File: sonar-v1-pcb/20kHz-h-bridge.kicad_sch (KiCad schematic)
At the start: 1 part, among them U34 DRV8876PWPR

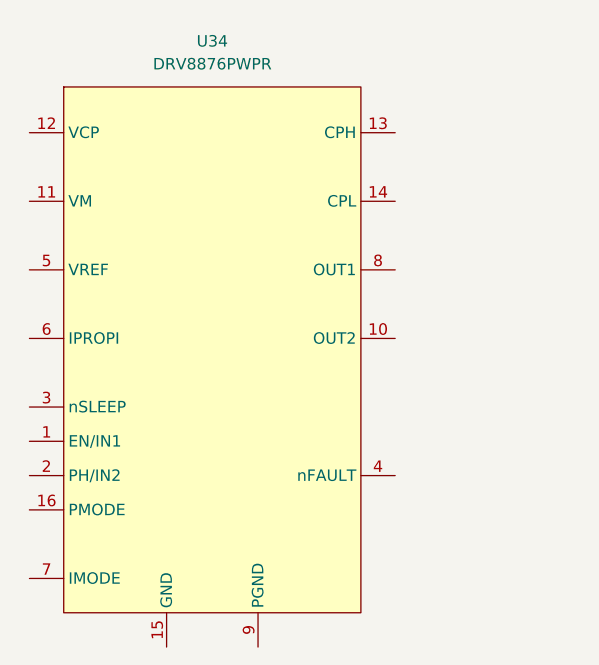
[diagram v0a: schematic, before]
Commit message: Do some power work
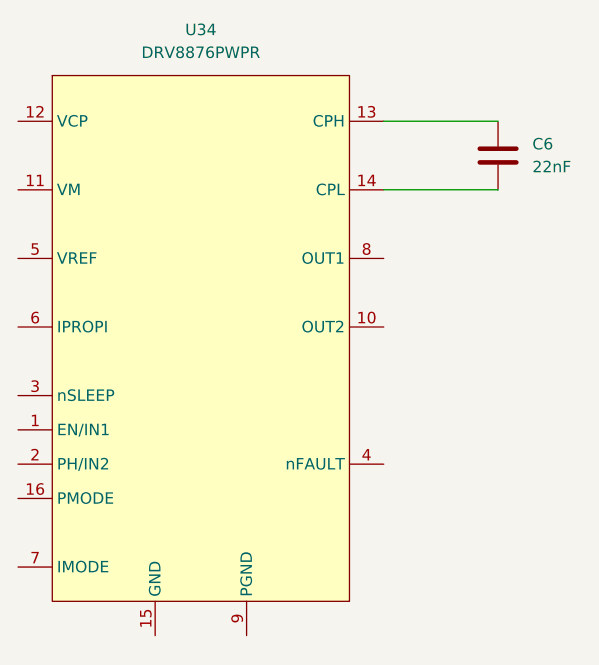
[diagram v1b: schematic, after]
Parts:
- added C6: 22nF, GS_Capacitors:C_0603_1608Metric, symbol GS_Capacitor_0603:C_0603_22nF
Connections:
- net at U34.13 (CPH): now also C6.1
- net at U34.14 (CPL): now also C6.2
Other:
- moved on the sheet: U34
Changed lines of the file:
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@@
 		(comment 1 "George Sleen")
+	)
+	(wire
+		(pts
+			(xy 180.34 86.36) (xy 167.64 86.36)
+		)
+		(stroke
+			(width 0)
+			(type default)
+		)
+	)
+	(wire
+		(pts
+			(xy 180.34 78.74) (xy 167.64 78.74)
+		)
+		(stroke
+			(width 0)
+			(type default)
+		)
 	)
 	(symbol
 		(lib_id "GS_H_Bridges:DRV8876PWPR")
-		(at 148.59 104.14 0)
+		(at 147.32 102.87 0)
 		(unit 1)
 		(body_style 1)
@@
 		(fields_autoplaced yes)
 		(property "Reference" "U34"
-			(at 148.59 69.85 0)
+			(at 147.32 68.58 0)
 			(show_name no)
 			(do_not_autoplace no)
@@
 		)
 		(property "Value" "DRV8876PWPR"
-			(at 148.59 72.39 0)
+			(at 147.32 71.12 0)
 			(show_name no)
 			(do_not_autoplace no)
@@
 		)
 		(property "Footprint" "GS_SO:HTSSOP-16-1EP_4.4x5mm_P0.65mm_EP3.4x5mm_Mask2.46x2.31mm"
-			(at 148.59 53.34 0)
+			(at 147.32 52.07 0)
 			(hide yes)
 			(show_name no)
@@
 		)
 		(property "Datasheet" "https://lcsc.com/product-detail/Motor-Drivers_Texas-Instruments-Texas-Instruments-DRV8876PWPR_C575551.html"
-			(at 148.59 43.18 0)
+			(at 147.32 41.91 0)
 			(hide yes)
 			(show_name no)
@@
 		)
 		(property "Description" "H-Bridge wih Integrated Current Sense and Regulation, 4.5V - 37V Input Voltage Range, 6A Max Current"
-			(at 148.59 45.72 0)
+			(at 147.32 44.45 0)
 			(hide yes)
 			(show_name no)
@@
 		)
 		(property "Manufacturer" "TI"
-			(at 148.59 40.64 0)
+			(at 147.32 39.37 0)
 			(hide yes)
 			(show_name no)
@@
 		)
 		(property "MPN" "DRV8876PWPR"
-			(at 148.59 50.8 0)
+			(at 147.32 49.53 0)
 			(hide yes)
 			(show_name no)
@@
 		)
 		(property "LCSC ID" "C575551"
-			(at 148.59 55.88 0)
+			(at 147.32 54.61 0)
 			(hide yes)
 			(show_name no)
@@
 		)
 		(property "Package" "HTSSOP-16_L5.0-W4.4-P0.65-LS6.4-BL-EP"
-			(at 148.59 48.26 0)
+			(at 147.32 46.99 0)
 			(hide yes)
 			(show_name no)
@@
 					(unit 1)
 				)
+			)
+		)
+	)
+	(symbol
+		(lib_id "GS_Capacitor_0603:C_0603_22nF")
+		(at 180.34 82.55 0)
+		(unit 1)
+		(body_style 1)
+		(exclude_from_sim no)
+		(in_bom yes)
+		(on_board yes)
+		(in_pos_files yes)
+		(dnp no)
+		(fields_autoplaced yes)
+		(property "Reference" "C6"
+			(at 184.15 81.2799 0)
+			(show_name no)
+			(do_not_autoplace no)
+			(effects
+				(font
+					(size 1.27 1.27)
+				)
+				(justify left)
+			)
+		)
+		(property "Value" "22nF"
+			(at 184.15 83.8199 0)
+			(show_name no)
+			(do_not_autoplace no)
+			(effects
+				(font
+					(size 1.27 1.27)
+				)
+				(justify left)
+			)
+		)
+		(property "Footprint" "GS_Capacitors:C_0603_1608Metric"
+			(at 180.34 60.198 0)
+			(hide yes)
+			(show_name no)
+			(do_not_autoplace no)
+			(effects
+				(font
+					(size 1.27 1.27)
+				)
+			)
+		)
+		(property "Datasheet" "https://datasheet.lcsc.com/datasheet/pdf/02336ea48ea44ca18c72517dd3cb7b47.pdf?productCode=C21122"
+			(at 180.34 68.834 0)
+			(hide yes)
+			(show_name no)
+			(do_not_autoplace no)
+			(effects
+				(font
+					(size 1.27 1.27)
+				)
+			)
+		)
+		(property "Description" "22nF 10% Unpolarized Capacitor, 50V Max Voltage, X7R"
+			(at 180.34 66.802 0)
+			(hide yes)
+			(show_name no)
+			(do_not_autoplace no)
+			(effects
+				(font
+					(size 1.27 1.27)
+				)
+			)
+		)
+		(property "Manufacturer" "Samsung Electro-Mechanics"
+			(at 180.34 63.5 0)
+			(hide yes)
+			(show_name no)
+			(do_not_autoplace no)
+			(effects
+				(font
+					(size 1.27 1.27)
+				)
+			)
+		)
+		(property "MPN" "CL10B223KB8NNNC"
+			(at 180.34 65.278 0)
+			(hide yes)
+			(show_name no)
+			(do_not_autoplace no)
+			(effects
+				(font
+					(size 1.27 1.27)
+				)
+			)
+		)
+		(property "LCSC ID" "C21122"
+			(at 180.34 70.612 0)
+			(hide yes)
+			(show_name no)
+			(do_not_autoplace no)
+			(effects
+				(font
+					(size 1.27 1.27)
+				)
+			)
+		)
+		(property "Package" "0603"
+			(at 180.34 61.976 0)
+			(hide yes)
+			(show_name no)
+			(do_not_autoplace no)
+			(effects
+				(font
+					(size 1.27 1.27)
+				)
+			)
+		)
+		(pin "2"
+		)
+		(pin "1"
+		)
+		(instances
+			(project "sonar"
+				(path "/f72ceae0-eee4-4385-b0e8-639846bcb5f2/c6a046af-5387-4c6b-a77e-149ae78eccdc"
+					(reference "C6")
+					(unit 1)
+				)
